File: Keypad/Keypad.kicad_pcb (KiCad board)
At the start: 2 copper layers, 41 parts, among them SW1 SW_Push, SW10 SW_Push, SW11 SW_Push, SW12 SW_Push, SW13 SW_Push, SW14 SW_Push, SW15 SW_Push, SW16 SW_Push, SW2 SW_Push, SW3 SW_Push, SW4 SW_Push, SW5 SW_Push, SW6 SW_Push, SW7 SW_Push, SW8 SW_Push, SW9 SW_Push

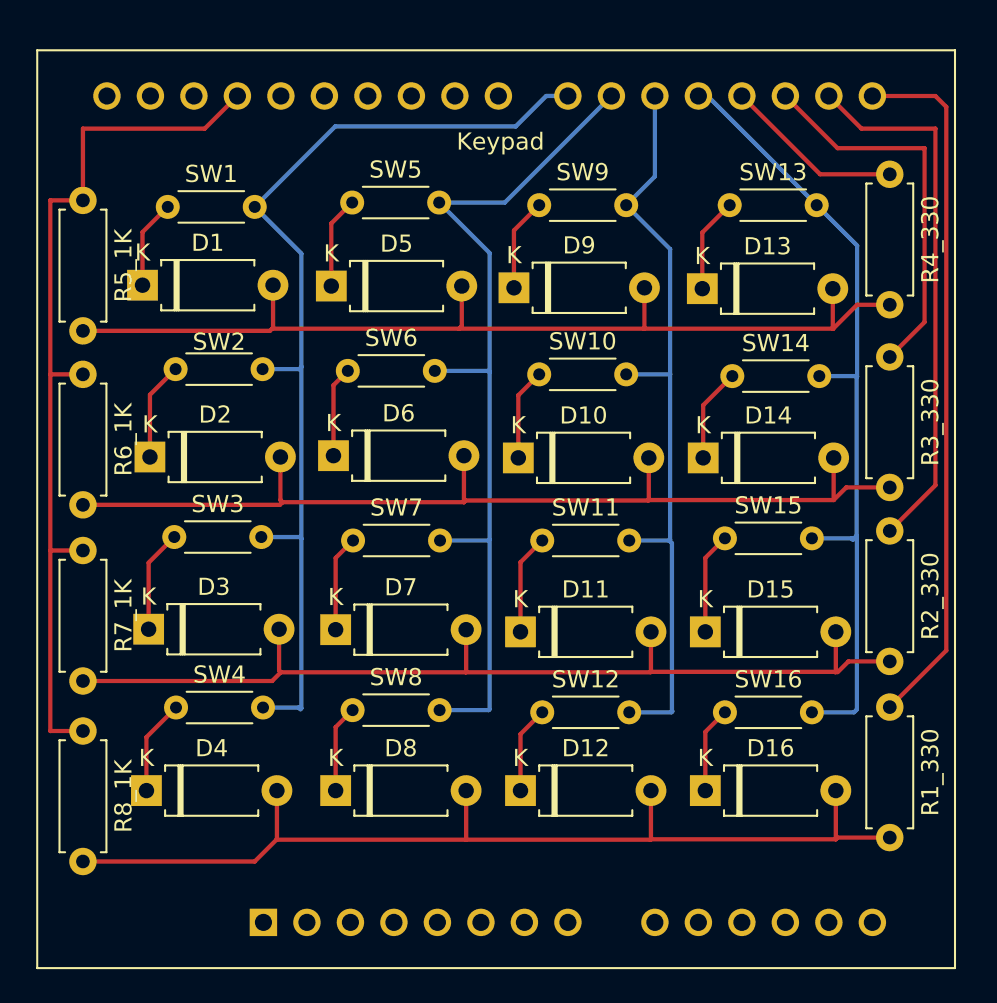
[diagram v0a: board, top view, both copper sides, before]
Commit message: Working on de10lite keypad 2.0
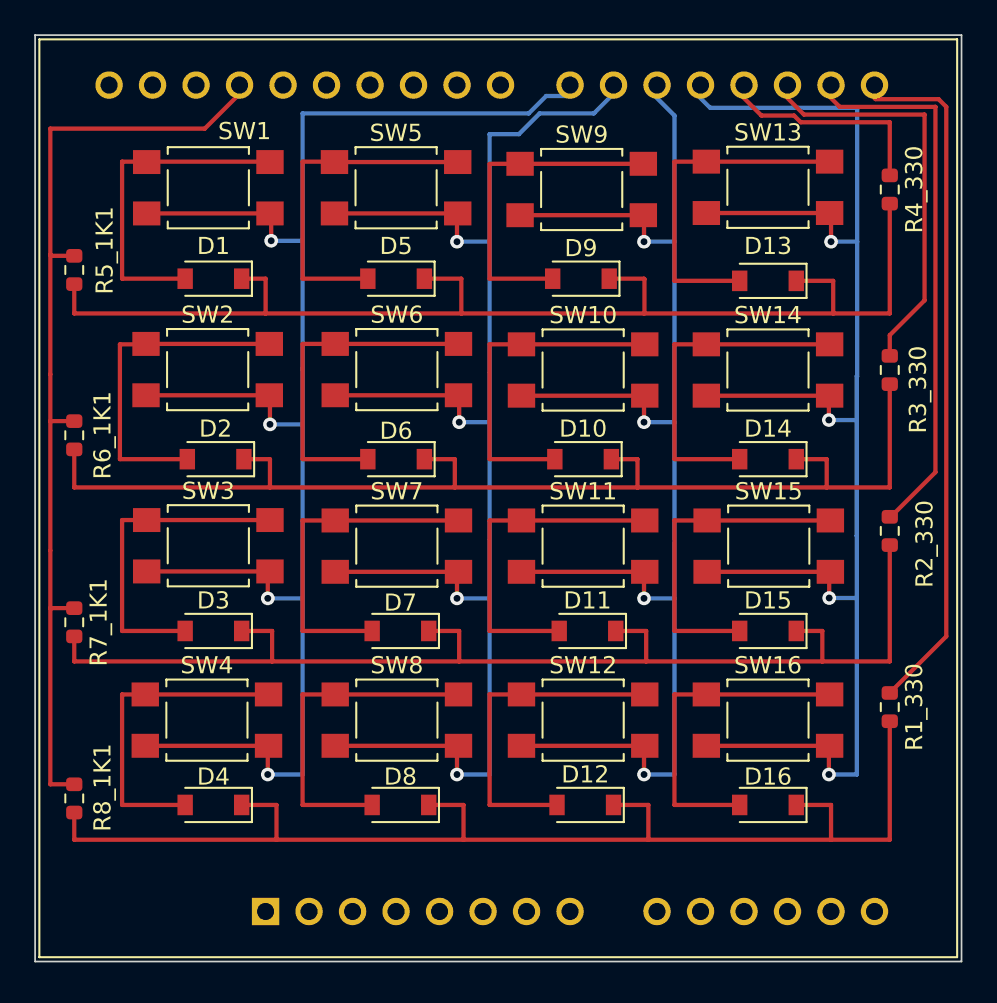
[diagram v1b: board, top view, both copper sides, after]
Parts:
- removed R6_1K, R7_1K, R8_1K: R_Small_US, Resistor_THT:R_Axial_DIN0207_L6.3mm_D2.5mm_P7.62mm_Horizontal
- added R6_1K1: R_Small_US, Resistor_SMD:R_0603_1608Metric, F.Cu at (113.2, 66.5)
- added R7_1K1: R_Small_US, Resistor_SMD:R_0603_1608Metric, F.Cu at (113.2, 77.5)
- added R8_1K1: R_Small_US, Resistor_SMD:R_0603_1608Metric, F.Cu at (113.2, 87.8)
- D1, D10, D11, D12, D13, D14, D15, D16, D2, D3, D4, D5, D6, D7, D8, D9: footprint Diode_THT:D_A-405_P7.62mm_Horizontal -> Diode_SMD:D_SOD-123
- R1_330, R2_330, R3_330, R4_330: footprint Resistor_THT:R_Axial_DIN0207_L6.3mm_D2.5mm_P7.62mm_Horizontal -> Resistor_SMD:R_0603_1608Metric
- R5_1K1: renamed from R5_1K; footprint Resistor_THT:R_Axial_DIN0207_L6.3mm_D2.5mm_P7.62mm_Horizontal -> Resistor_SMD:R_0603_1608Metric
- SW1, SW10, SW11, SW12, SW13, SW14, SW15, SW16, SW2, SW3, SW4, SW5, SW6, SW7, SW8, SW9: footprint Resistor_THT:R_Axial_DIN0204_L3.6mm_D1.6mm_P5.08mm_Horizontal -> Button_Switch_SMD:SW_SPST_TL3305B
- moved D1 4.16 mm to (121.3, 57.4), turned to 180 degrees
- moved R5_1K1 4.10 mm to (113.2, 56.9)
- moved D4 4.00 mm to (121.3, 88.1), turned to 180 degrees
- moved D9 3.95 mm to (142.7, 57.4), turned to 180 degrees
- moved D11 3.91 mm to (143.1, 78.0), turned to 180 degrees
- moved D12 3.88 mm to (143.0, 88.1), turned to 180 degrees
- moved D8 3.88 mm to (132.2, 88.1), turned to 180 degrees
- moved D13 3.86 mm to (153.7, 57.5), turned to 180 degrees
- moved D2 3.84 mm to (121.4, 67.9), turned to 180 degrees
- moved D5 3.81 mm to (132.0, 57.4), turned to 180 degrees
- moved D3 3.79 mm to (121.3, 78.0), turned to 180 degrees
- moved D10 3.79 mm to (142.9, 67.9), turned to 180 degrees
- moved D14 3.79 mm to (153.7, 67.9), turned to 180 degrees
- moved D7 3.79 mm to (132.2, 78.0), turned to 180 degrees
- moved D16 3.75 mm to (153.7, 88.1), turned to 180 degrees
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- renumbered Keypad to U1
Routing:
- net Net-(SW13-Pad2): track 47.7 -> 90.1 mm, vias 0 -> 4
- net Net-(SW1-Pad2): track 58.4 -> 97.9 mm, vias 0 -> 4
- net Net-(SW10-Pad2): track 45.2 -> 82.3 mm, vias 0 -> 4
- net Net-(SW5-Pad2): track 52.5 -> 88.3 mm, vias 0 -> 4
- net Net-(D8-Pad1): track 5.11 -> 19.6 mm
- net Net-(D12-Pad1): track 5.10 -> 19.5 mm
- net Net-(D6-Pad1): track 5.30 -> 19.6 mm
- net Net-(D5-Pad1): track 5.38 -> 19.7 mm
- net Net-(D13-Pad1): track 5.54 -> 19.8 mm
- net Net-(D16-Pad1): track 5.05 -> 19.3 mm
- net Net-(D10-Pad1): track 5.38 -> 19.6 mm
- net Net-(D9-Pad1): track 5.44 -> 19.6 mm
- net Net-(D14-Pad1): track 5.48 -> 19.6 mm
- net Net-(D1-Pad1): track 5.18 -> 19.2 mm
- net Net-(D7-Pad1): track 5.63 -> 19.6 mm
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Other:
- board outline added: 54.1 x 54.1 mm
- copper layers 2 -> 4
